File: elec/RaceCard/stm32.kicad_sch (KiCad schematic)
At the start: 14 parts, among them J1 Conn_ST_STDC14, U1 STM32U031C6Tx

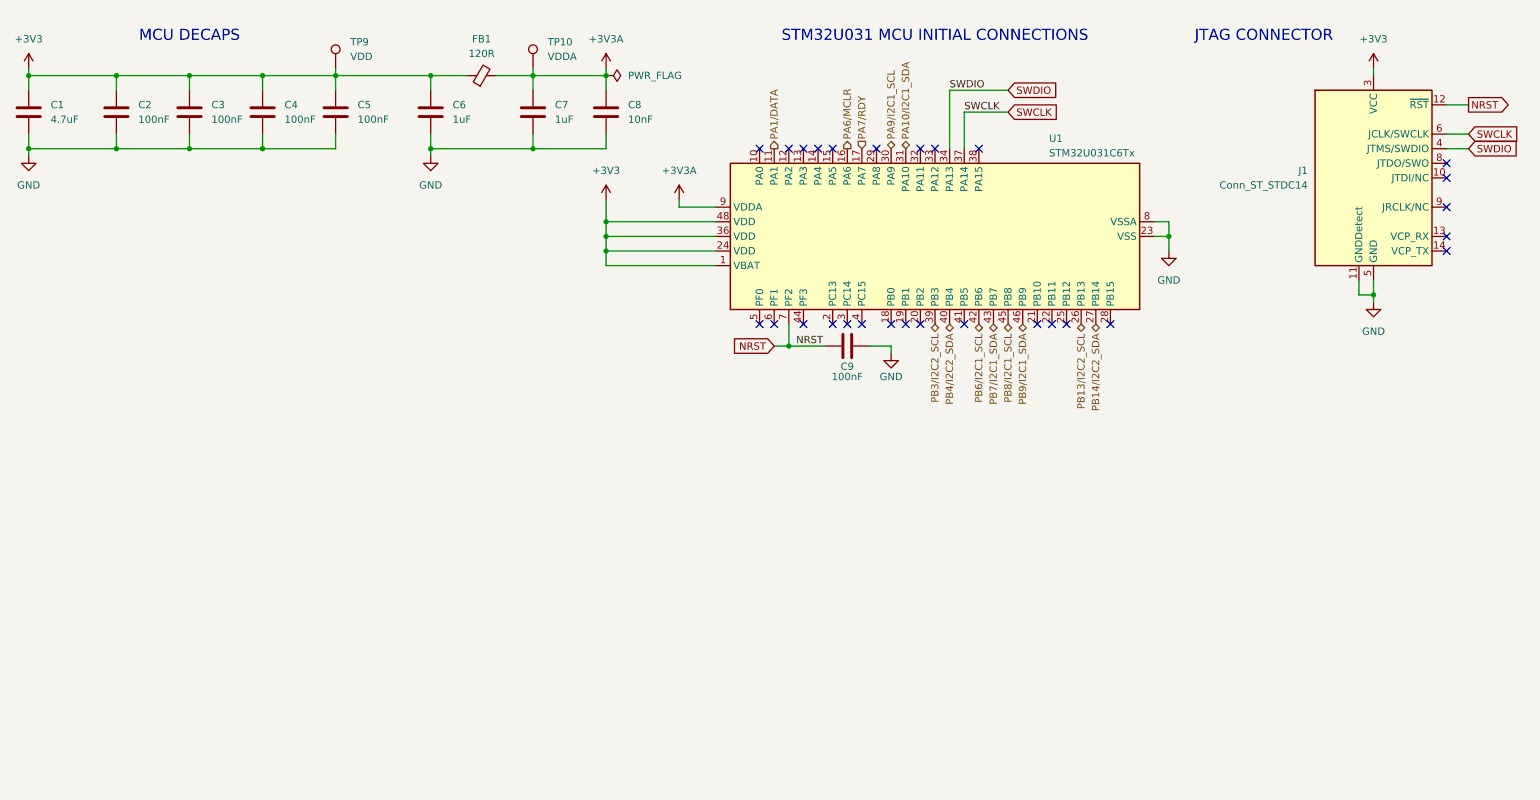
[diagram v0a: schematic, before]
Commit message: Cleanup
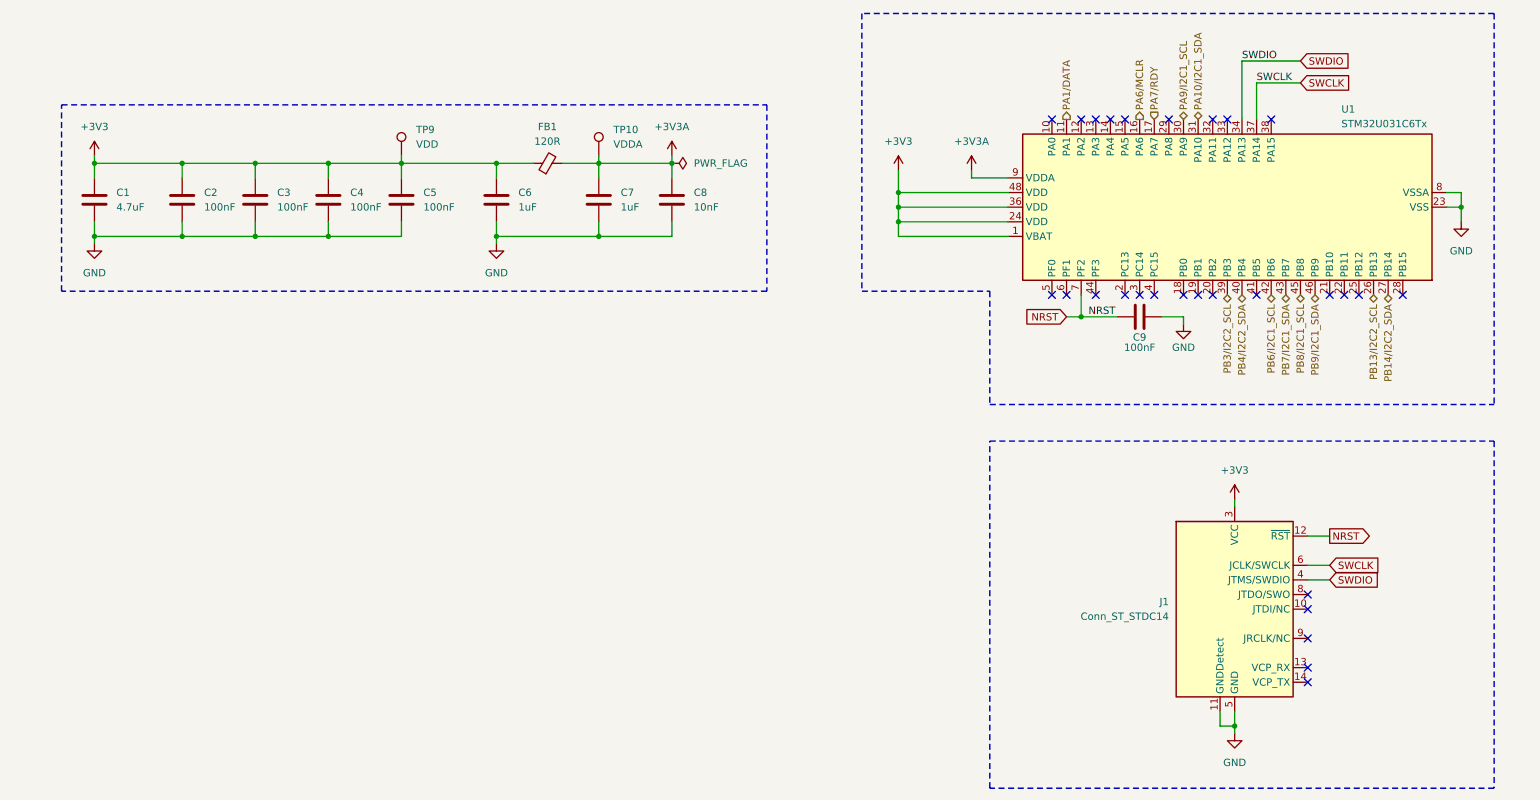
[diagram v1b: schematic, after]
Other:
- note removed: "JTAG CONNECTOR"
- note removed: "MCU DECAPS"
- note removed: "STM32U031 MCU INITIAL CONNECTIONS"
- moved on the sheet: C1, C2, C3, C4, C5, C6, C7, C8, C9, FB1, J1, TP10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
